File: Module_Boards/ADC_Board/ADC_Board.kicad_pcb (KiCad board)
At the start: 6 copper layers, 15.6 x 19.7 mm, 74 parts, among them J1 212134-0003, J2 212134-0003, J3 212134-0003, J4 212134-0003, U1 ADS8860IDRCT, U2 REF35250YBHR, U3 TPS22916CYFPR, U4 TPS7A9401DSCR, U5 TMUX1104DQAR, U6 LTC6255IDC#TRMPBF, U7 OPA310SIDBVR, U8 OPA333AIDBVR

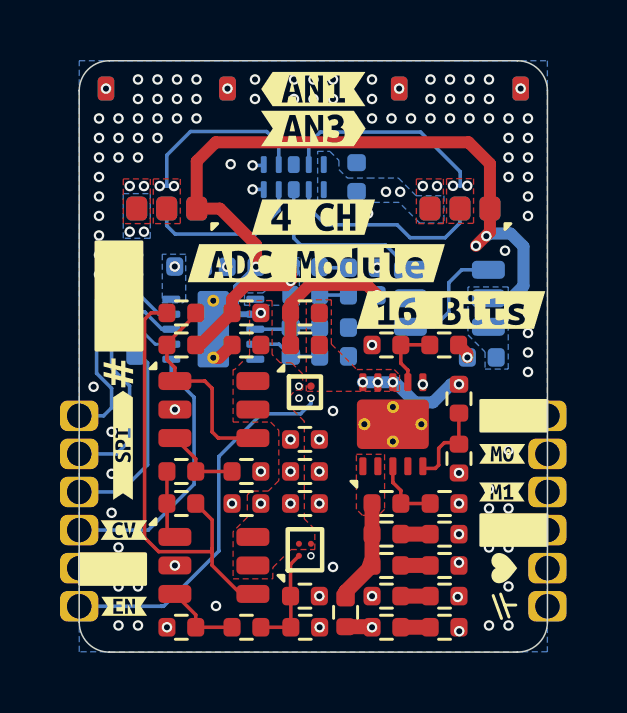
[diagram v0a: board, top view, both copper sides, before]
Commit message: Final revision and production files
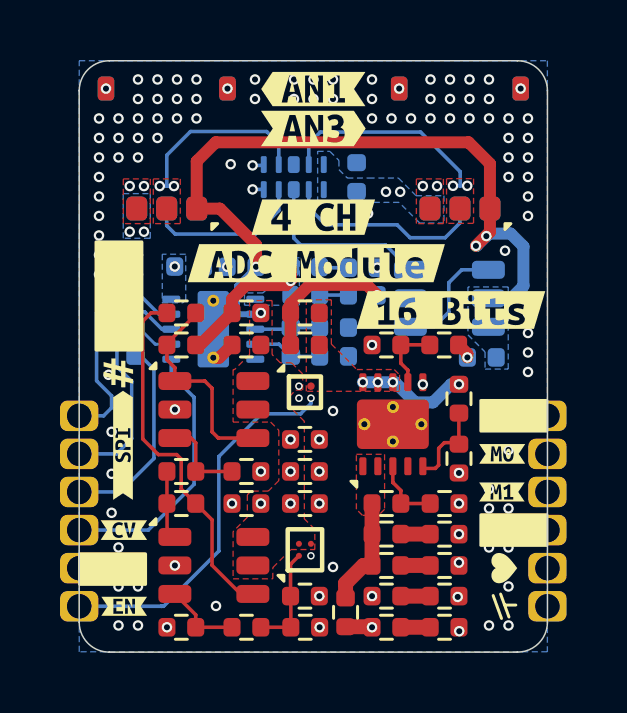
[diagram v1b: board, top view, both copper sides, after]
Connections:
- net /[1] Power Regulation & Level Shifting/+3V3_FILT renamed /[1] Power Regulation & Connectors/+3V3_FILT
- net /[1] Power Regulation & Level Shifting/EN_UV renamed /[1] Power Regulation & Connectors/EN_UV
- net /[1] Power Regulation & Level Shifting/FB_PG renamed /[1] Power Regulation & Connectors/FB_PG
- net /[1] Power Regulation & Level Shifting/NR/SS renamed /[1] Power Regulation & Connectors/NR/SS
- net /[2] ADC & Multiplexer/ADC_IN_N renamed /[2] ADC, Multiplexer & Reference/ADC_IN_N
- net /[2] ADC & Multiplexer/ADC_IN_P renamed /[2] ADC, Multiplexer & Reference/ADC_IN_P
- net /[2] ADC & Multiplexer/AN_1 renamed /[2] ADC, Multiplexer & Reference/AN_1
- net /[2] ADC & Multiplexer/AN_2 renamed /[2] ADC, Multiplexer & Reference/AN_2
- net /[2] ADC & Multiplexer/AN_3 renamed /[2] ADC, Multiplexer & Reference/AN_3
- net /[2] ADC & Multiplexer/AN_4 renamed /[2] ADC, Multiplexer & Reference/AN_4
- net /[2] ADC & Multiplexer/BUFFER_IN renamed /[2] ADC, Multiplexer & Reference/BUFFER_IN
- net /[2] ADC & Multiplexer/CHARGE_BUCKET_IN renamed /[2] ADC, Multiplexer & Reference/CHARGE_BUCKET_IN
- net /[2] ADC & Multiplexer/REF_OUT renamed /[2] ADC, Multiplexer & Reference/REF_OUT
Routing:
- net Net-(U8--): track 14.7 -> 12.1 mm
- net GND: vias 137 -> 136
